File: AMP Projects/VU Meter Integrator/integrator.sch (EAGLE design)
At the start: 28 parts, among them IC1 OPAMP-DUALDIP

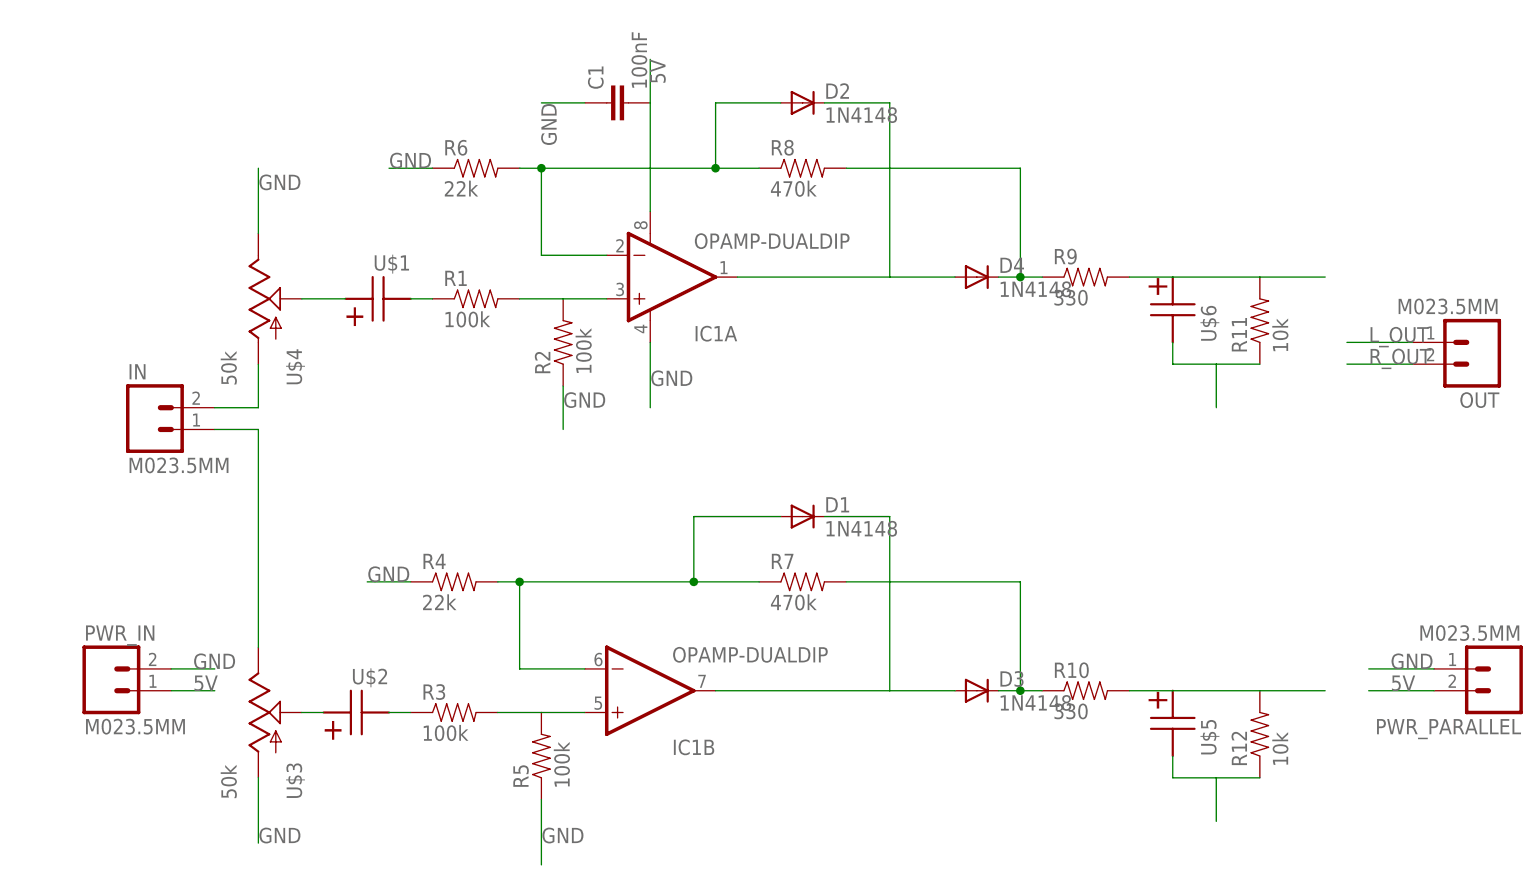
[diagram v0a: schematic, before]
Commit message: Updates to most boards
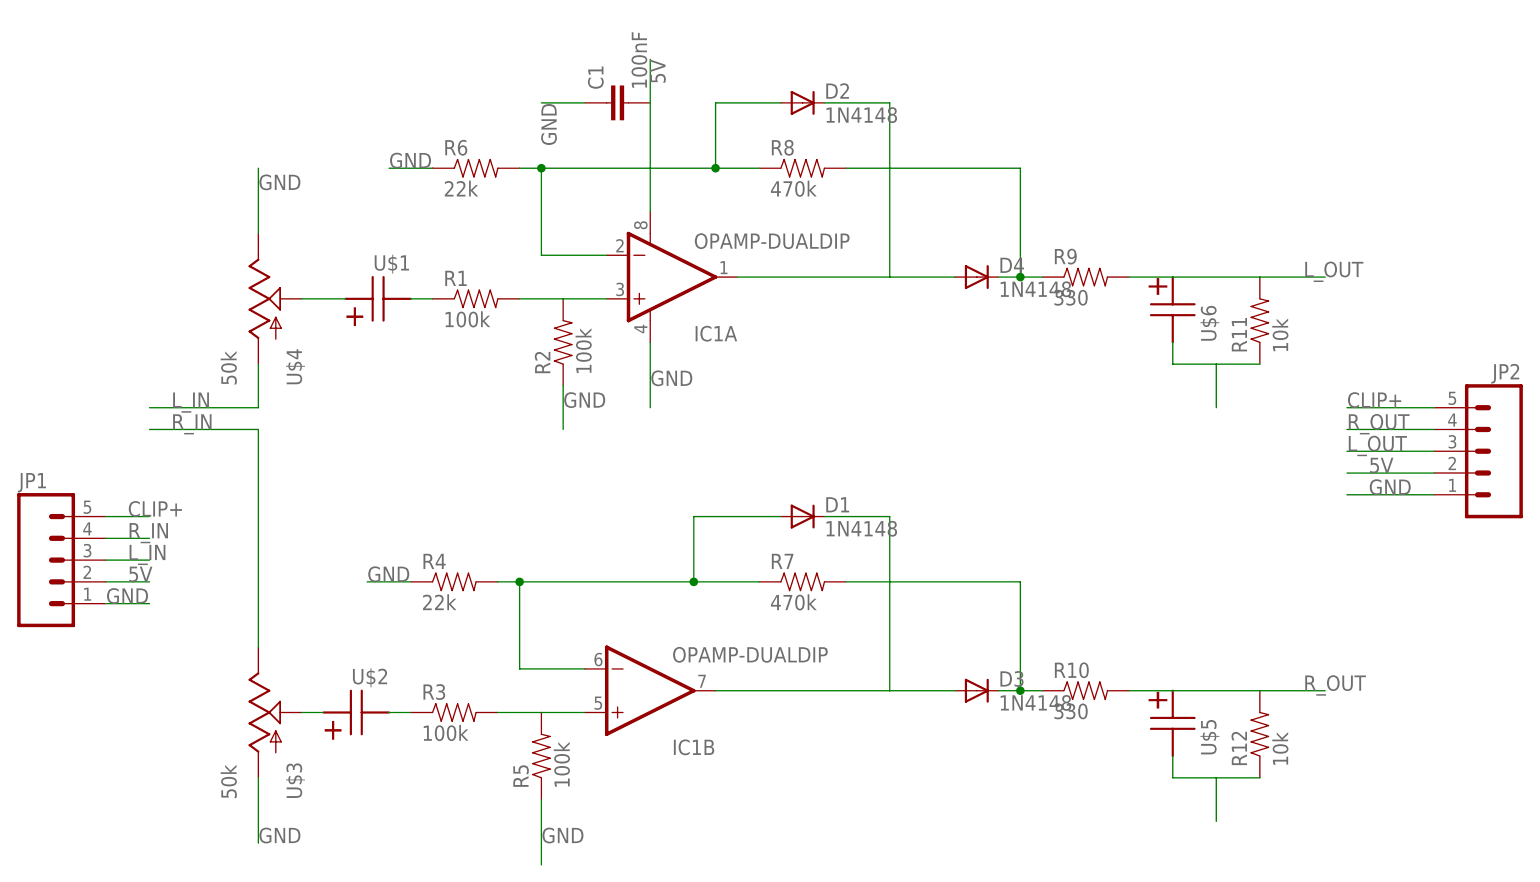
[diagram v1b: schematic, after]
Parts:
- removed IN, OUT, PWR_IN, PWR_PARALLEL: M023.5MM, SparkFun-Connectors:M023.5MM
- added JP1, JP2: (no value), SparkFun-Connectors:M05SMD2
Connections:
- new net CLIP+: JP1.5, JP2.5
- net 5V: now also JP1.2, JP2.2; no longer PWR_IN.1, PWR_PARALLEL.2
- net GND: now also JP1.1, JP2.1; no longer PWR_IN.2, PWR_PARALLEL.1
- net L_IN: now also JP1.3; no longer IN.2
- net L_OUT: now also JP2.3; no longer OUT.1
- net R_IN: now also JP1.4; no longer IN.1
- net R_OUT: now also JP2.4; no longer OUT.2
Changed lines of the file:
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@@
 <?xml version="1.0" encoding="utf-8"?>
 <!DOCTYPE eagle SYSTEM "eagle.dtd">
-<eagle version="6.5.0">
+<eagle version="7.1.0">
 <drawing>
 <settings>
@@
 <part name="D3" library="SparkFun-DiscreteSemi" deviceset="DIODE" device="1N4148" value="1N4148"/>
 <part name="D4" library="SparkFun-DiscreteSemi" deviceset="DIODE" device="1N4148" value="1N4148"/>
-<part name="IN" library="SparkFun-Connectors" deviceset="M02" device="3.5MM"/>
-<part name="PWR_IN" library="SparkFun-Connectors" deviceset="M02" device="3.5MM"/>
-<part name="OUT" library="SparkFun-Connectors" deviceset="M02" device="3.5MM"/>
-<part name="PWR_PARALLEL" library="SparkFun-Connectors" deviceset="M02" device="3.5MM"/>
 <part name="U$1" library="AMP Library" deviceset="5MM-12.5MM-POLAR" device="2MMX5MM" value="6.8uF"/>
 <part name="U$2" library="AMP Library" deviceset="5MM-12.5MM-POLAR" device="2MMX5MM" value="6.8uF"/>
 <part name="U$5" library="AMP Library" deviceset="5MM-12.5MM-POLAR" device="2MMX5MM" value="2.2uF"/>
 <part name="U$6" library="AMP Library" deviceset="5MM-12.5MM-POLAR" device="2MMX5MM" value="2.2uF"/>
+<part name="JP1" library="SparkFun-Connectors" deviceset="M05" device="SMD2"/>
+<part name="JP2" library="SparkFun-Connectors" deviceset="M05" device="SMD2"/>
 </parts>
 <sheets>
@@
 <instance part="D3" gate="G$1" x="71.12" y="20.32"/>
 <instance part="D4" gate="G$1" x="71.12" y="68.58"/>
-<instance part="IN" gate="G$1" x="-25.4" y="50.8"/>
-<instance part="PWR_IN" gate="G$1" x="-30.48" y="20.32"/>
-<instance part="OUT" gate="G$1" x="129.54" y="60.96" rot="R180"/>
-<instance part="PWR_PARALLEL" gate="G$1" x="132.08" y="22.86" rot="R180"/>
 <instance part="U$1" gate="G$1" x="0" y="66.04" rot="R180"/>
 <instance part="U$2" gate="G$1" x="-2.54" y="17.78" rot="R180"/>
 <instance part="U$5" gate="G$1" x="93.98" y="17.78" rot="R90"/>
 <instance part="U$6" gate="G$1" x="93.98" y="66.04" rot="R90"/>
+<instance part="JP1" gate="G$1" x="-38.1" y="35.56"/>
+<instance part="JP2" gate="G$1" x="132.08" y="48.26" rot="MR0"/>
 </instances>
 <busses>
@@
 <net name="R_IN" class="0">
 <segment>
-<pinref part="IN" gate="G$1" pin="1"/>
-<wire x1="-17.78" y1="50.8" x2="-12.7" y2="50.8" width="0.1524" layer="91"/>
+<wire x1="-25.4" y1="50.8" x2="-12.7" y2="50.8" width="0.1524" layer="91"/>
 <wire x1="-12.7" y1="50.8" x2="-12.7" y2="25.4" width="0.1524" layer="91"/>
 <pinref part="U$3" gate="G$1" pin="E"/>
+<label x="-22.86" y="50.8" size="1.778" layer="95"/>
+</segment>
+<segment>
+<pinref part="JP1" gate="G$1" pin="4"/>
+<wire x1="-30.48" y1="38.1" x2="-25.4" y2="38.1" width="0.1524" layer="91"/>
+<label x="-27.94" y="38.1" size="1.778" layer="95"/>
 </segment>
 </net>
@@
 <net name="L_IN" class="0">
 <segment>
-<pinref part="IN" gate="G$1" pin="2"/>
-<wire x1="-17.78" y1="53.34" x2="-12.7" y2="53.34" width="0.1524" layer="91"/>
+<wire x1="-25.4" y1="53.34" x2="-12.7" y2="53.34" width="0.1524" layer="91"/>
 <wire x1="-12.7" y1="53.34" x2="-12.7" y2="58.42" width="0.1524" layer="91"/>
 <pinref part="U$4" gate="G$1" pin="A"/>
+<label x="-22.86" y="53.34" size="1.778" layer="95"/>
+</segment>
+<segment>
+<pinref part="JP1" gate="G$1" pin="3"/>
+<wire x1="-30.48" y1="35.56" x2="-25.4" y2="35.56" width="0.1524" layer="91"/>
+<label x="-27.94" y="35.56" size="1.778" layer="95"/>
 </segment>
 </net>
@@
 </segment>
 <segment>
-<pinref part="PWR_IN" gate="G$1" pin="2"/>
-<wire x1="-22.86" y1="22.86" x2="-17.78" y2="22.86" width="0.1524" layer="91"/>
-<label x="-20.32" y="22.86" size="1.778" layer="95"/>
-</segment>
-<segment>
-<pinref part="PWR_PARALLEL" gate="G$1" pin="1"/>
-<wire x1="124.46" y1="22.86" x2="116.84" y2="22.86" width="0.1524" layer="91"/>
-<label x="119.38" y="22.86" size="1.778" layer="95"/>
+<wire x1="-30.48" y1="30.48" x2="-25.4" y2="30.48" width="0.1524" layer="91"/>
+<label x="-30.48" y="30.48" size="1.778" layer="95"/>
+<pinref part="JP1" gate="G$1" pin="1"/>
+</segment>
+<segment>
+<wire x1="124.46" y1="43.18" x2="114.3" y2="43.18" width="0.1524" layer="91"/>
+<label x="116.84" y="43.18" size="1.778" layer="95"/>
+<pinref part="JP2" gate="G$1" pin="1"/>
 </segment>
 <segment>
@@
 <net name="5V" class="0">
 <segment>
-<pinref part="PWR_IN" gate="G$1" pin="1"/>
-<wire x1="-22.86" y1="20.32" x2="-17.78" y2="20.32" width="0.1524" layer="91"/>
-<label x="-20.32" y="20.32" size="1.778" layer="95"/>
-</segment>
-<segment>
-<pinref part="PWR_PARALLEL" gate="G$1" pin="2"/>
-<wire x1="124.46" y1="20.32" x2="116.84" y2="20.32" width="0.1524" layer="91"/>
-<label x="119.38" y="20.32" size="1.778" layer="95"/>
+<wire x1="-30.48" y1="33.02" x2="-25.4" y2="33.02" width="0.1524" layer="91"/>
+<label x="-27.94" y="33.02" size="1.778" layer="95"/>
+<pinref part="JP1" gate="G$1" pin="2"/>
+</segment>
+<segment>
+<wire x1="124.46" y1="45.72" x2="114.3" y2="45.72" width="0.1524" layer="91"/>
+<label x="116.84" y="45.72" size="1.778" layer="95"/>
+<pinref part="JP2" gate="G$1" pin="2"/>
 </segment>
 <segment>
@@
 <net name="L_OUT" class="0">
 <segment>
-<pinref part="OUT" gate="G$1" pin="1"/>
-<wire x1="121.92" y1="60.96" x2="114.3" y2="60.96" width="0.1524" layer="91"/>
-<label x="116.84" y="60.96" size="1.778" layer="95"/>
+<wire x1="124.46" y1="48.26" x2="114.3" y2="48.26" width="0.1524" layer="91"/>
+<label x="114.3" y="48.26" size="1.778" layer="95"/>
+<pinref part="JP2" gate="G$1" pin="3"/>
 </segment>
 <segment>
@@
 <wire x1="93.98" y1="68.58" x2="104.14" y2="68.58" width="0.1524" layer="91"/>
 <wire x1="104.14" y1="68.58" x2="111.76" y2="68.58" width="0.1524" layer="91"/>
+<label x="109.22" y="68.58" size="1.778" layer="95"/>
 </segment>
 </net>
 <net name="R_OUT" class="0">
 <segment>
-<pinref part="OUT" gate="G$1" pin="2"/>
-<wire x1="121.92" y1="58.42" x2="114.3" y2="58.42" width="0.1524" layer="91"/>
-<label x="116.84" y="58.42" size="1.778" layer="95"/>
+<wire x1="124.46" y1="50.8" x2="114.3" y2="50.8" width="0.1524" layer="91"/>
+<label x="114.3" y="50.8" size="1.778" layer="95"/>
+<pinref part="JP2" gate="G$1" pin="4"/>
 </segment>
 <segment>
@@
 <wire x1="93.98" y1="20.32" x2="104.14" y2="20.32" width="0.1524" layer="91"/>
 <wire x1="104.14" y1="20.32" x2="111.76" y2="20.32" width="0.1524" layer="91"/>
-</segment>
-</net>
+<label x="109.22" y="20.32" size="1.778" layer="95"/>
+</segment>
+</net>
+<net name="CLIP+" class="0">
+<segment>
+<pinref part="JP2" gate="G$1" pin="5"/>
+<wire x1="124.46" y1="53.34" x2="114.3" y2="53.34" width="0.1524" layer="91"/>
+<label x="114.3" y="53.34" size="1.778" layer="95"/>
+</segment>
+<segment>
+<pinref part="JP1" gate="G$1" pin="5"/>
+<wire x1="-30.48" y1="40.64" x2="-25.4" y2="40.64" width="0.1524" layer="91"/>
+<label x="-27.94" y="40.64" size="1.778" layer="95"/>
+</segment>
+</net>
